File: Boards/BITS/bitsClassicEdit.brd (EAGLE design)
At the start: 45 x 40 mm, 34 parts, among them T1 SI1013, U1 LMR16020, X2 53398-10

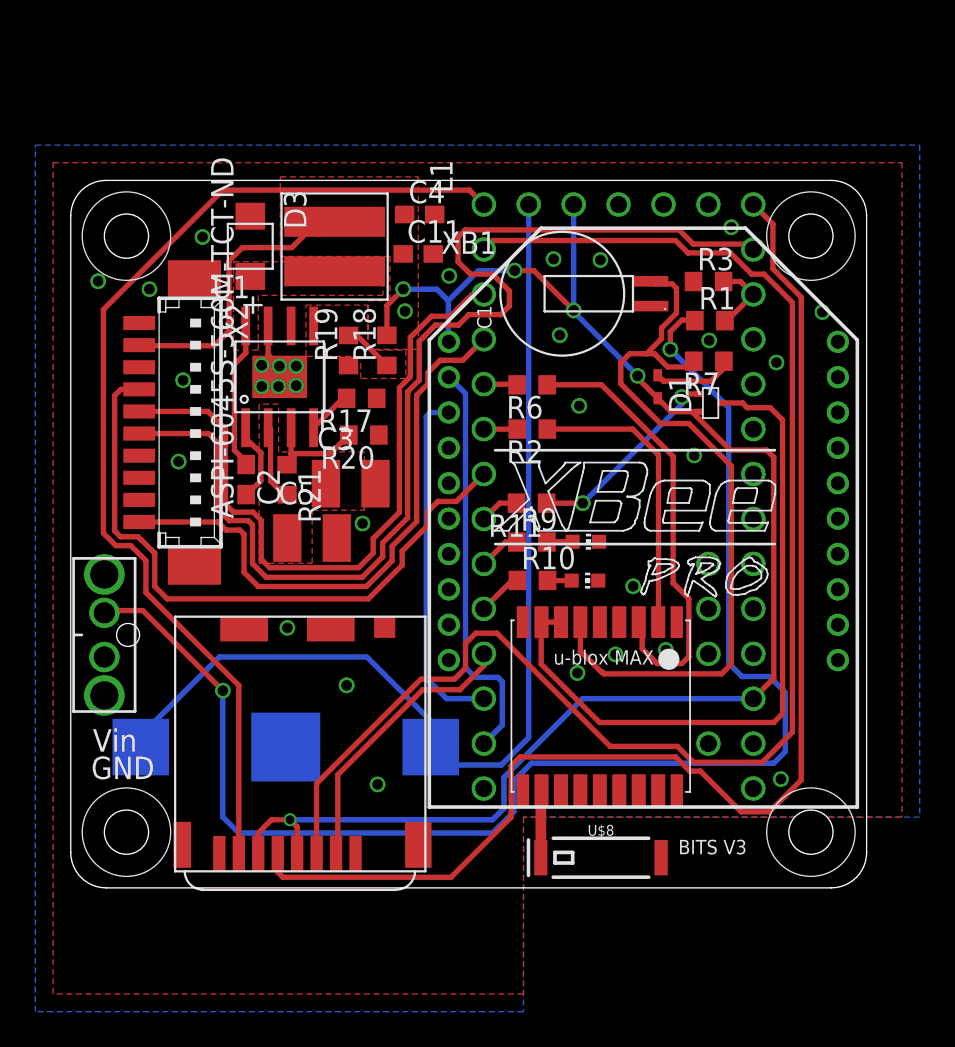
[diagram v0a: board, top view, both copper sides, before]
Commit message: Created an alternate board
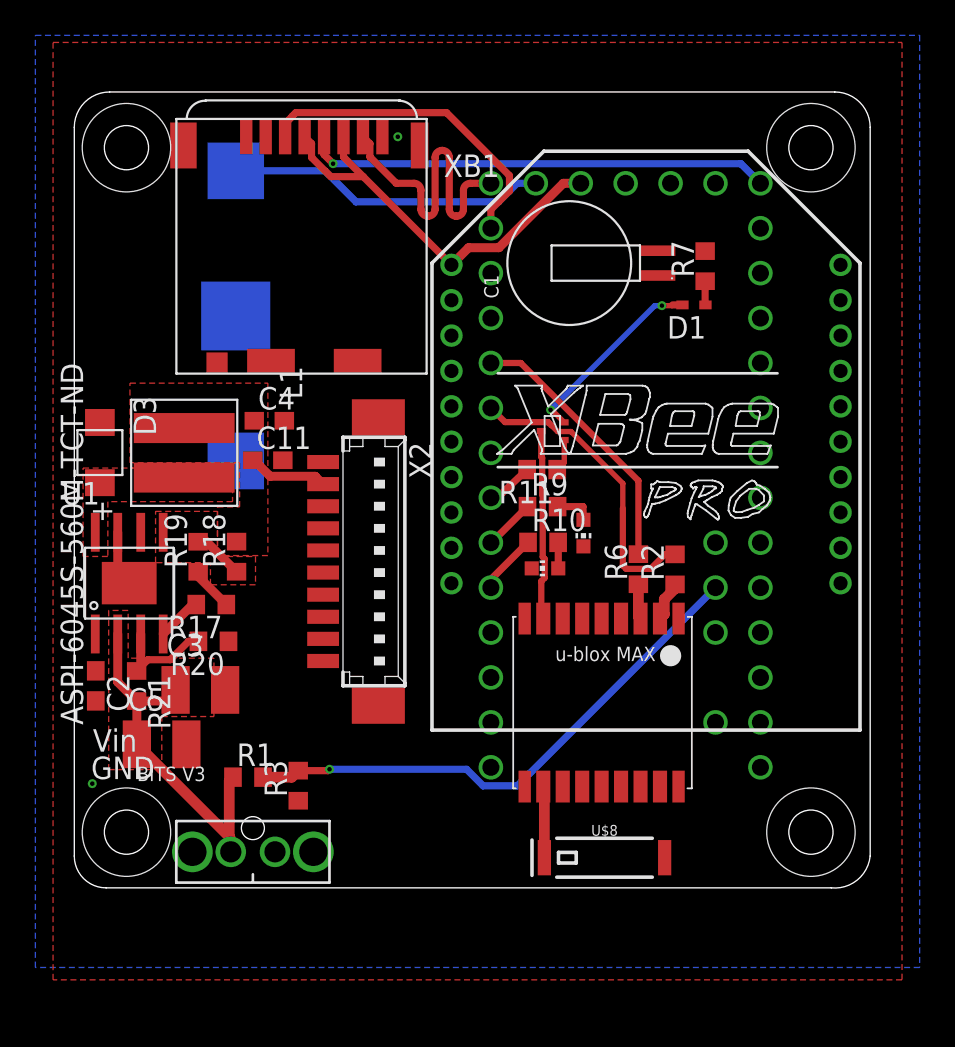
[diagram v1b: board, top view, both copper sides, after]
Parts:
- moved R3 36.8 mm to (12.9, 5.78), turned to 90 degrees
- moved R1 36.7 mm to (10.0, 6.26)
- moved U$3 24.5 mm to (9.33, 32.3), turned to 270 degrees
- moved U$4 15.1 mm to (9.92, 29.1), turned to 180 degrees
- moved U$1 14.9 mm to (10.3, 2.04), turned to 180 degrees
- moved C4 14.4 mm to (11.2, 26.4)
- moved D3 14.4 mm to (1.65, 24.6)
- moved R18 14.4 mm to (9.38, 18.7)
- moved C5 14.4 mm to (5.14, 8.12)
- moved C11 14.4 mm to (11.1, 24.2)
- moved C2 14.4 mm to (1.42, 11.4)
- moved C3 14.4 mm to (7.33, 11.2)
- moved L1 14.4 mm to (6.42, 24.6)
- moved R17 14.4 mm to (7.95, 16.0)
- moved R19 14.4 mm to (7.20, 18.7)
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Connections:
- removed net N$37: U$2.A10
- net BAT_CELL1: now also U$2.A10; no longer U$2.15/A1
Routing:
- net +3V3: track 103.9 -> 39.2 mm, vias 5 -> 2
- net MOSI: track 82.3 -> 18.6 mm
- net IN1: track 84.2 -> 20.9 mm, vias 2 -> 0
- net RING: track 63.2 -> 0.00 mm
- net SCK: track 71.0 -> 26.4 mm, vias 0 -> 1
- net V_BCKP: track 42.3 -> 0.00 mm
- net MISO: track 59.1 -> 18.1 mm
- net VBAT: track 58.7 -> 18.1 mm
- net TXD: track 39.2 -> 0.00 mm
- net SLEEP: track 36.6 -> 0.00 mm
- net RXD: track 33.1 -> 0.00 mm
- net N$11: track 39.2 -> 10.8 mm
- net BAT_CELL1: track 4.20 -> 30.8 mm, vias 0 -> 1
- net N$3: track 25.2 -> 1.99 mm
- net DOUT: track 23.2 -> 0.00 mm
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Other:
- board size 45 x 40 mm -> 45 x 45 mm
